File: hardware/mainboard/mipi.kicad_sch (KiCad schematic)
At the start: 41 parts

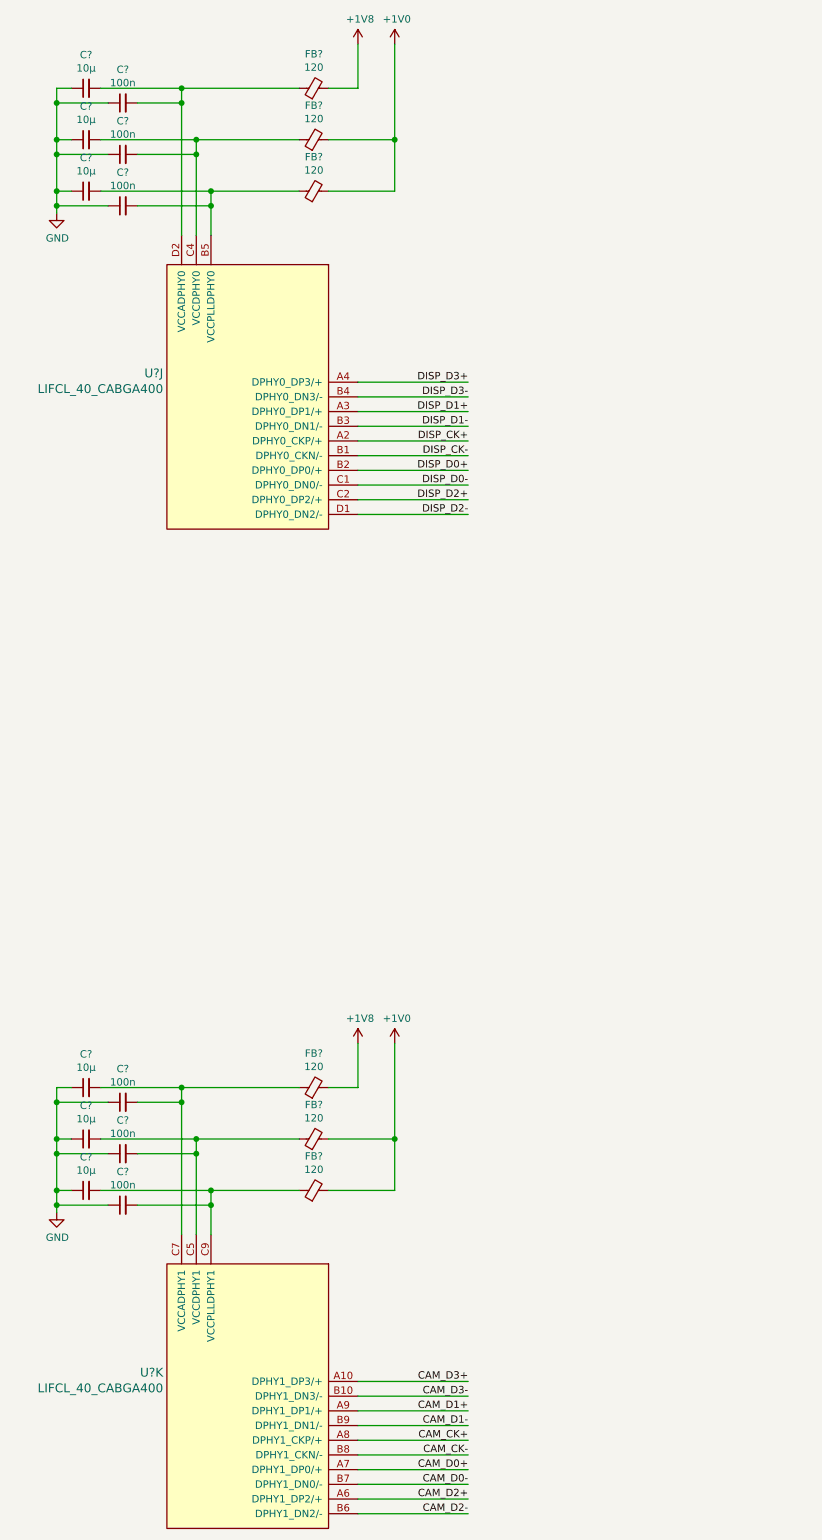
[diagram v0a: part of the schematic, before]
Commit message: More stuff
Signed-off-by: David Shah <dave@ds0.me>
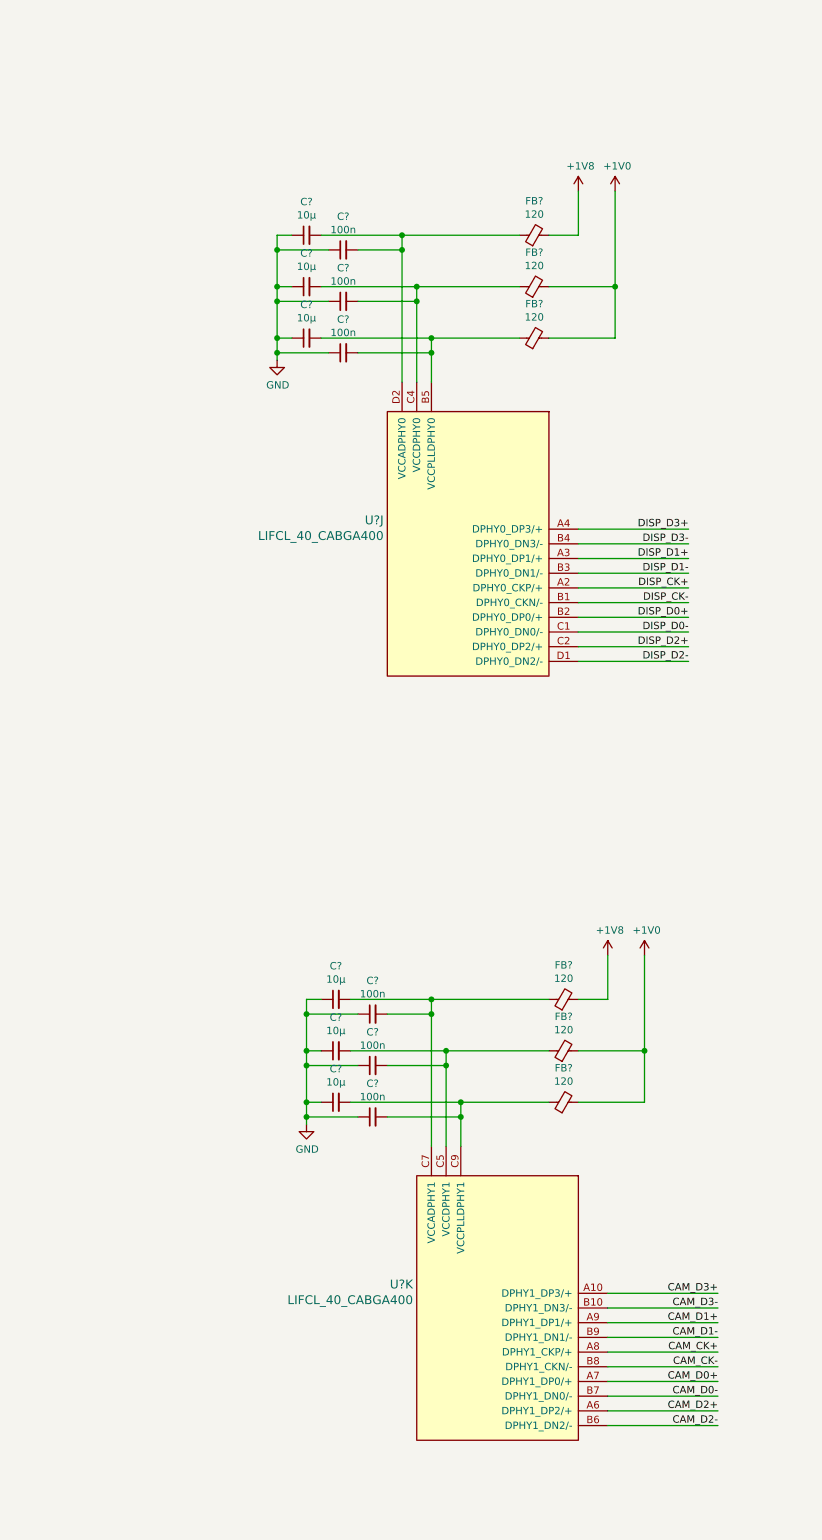
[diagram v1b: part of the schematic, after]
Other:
- moved on the sheet: C?, FB?, U?J, U?K
